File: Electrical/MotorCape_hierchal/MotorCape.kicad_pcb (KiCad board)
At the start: 2 copper layers, 24 parts, among them J1 Motor1, J10 DualMotorController_SIG, J11 flag_wheel servo, J12 Motor2, J13 Motor1, J14 DualMotorController_PWR, J16 DualMotorController_SIG, J17 Motor2, J2 DualMotorController_PWR, J4 DualMotorController_SIG, J5 Motor2, J6 Motor1, J7 i2c bus connector, J8 DualMotorController_PWR, P13 battery_connector, P14 Pi_Connector, U1 IMU

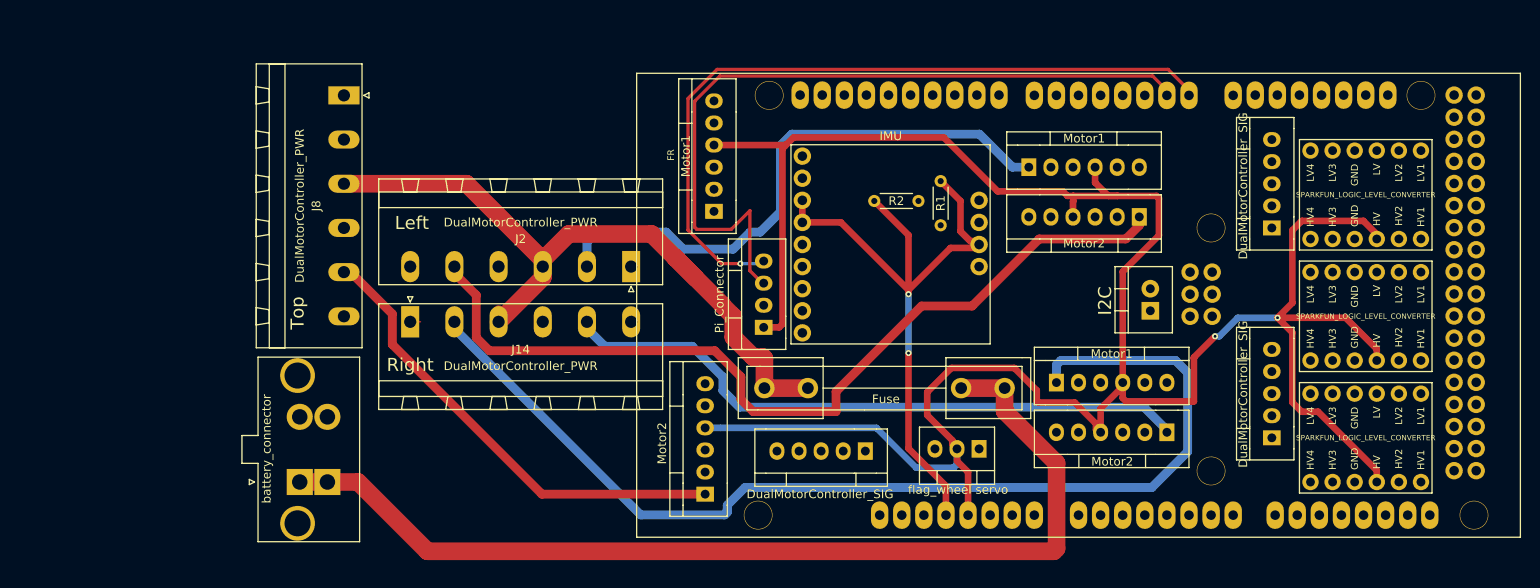
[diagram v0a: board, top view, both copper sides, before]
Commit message: pushing changes while routing. still not done yet
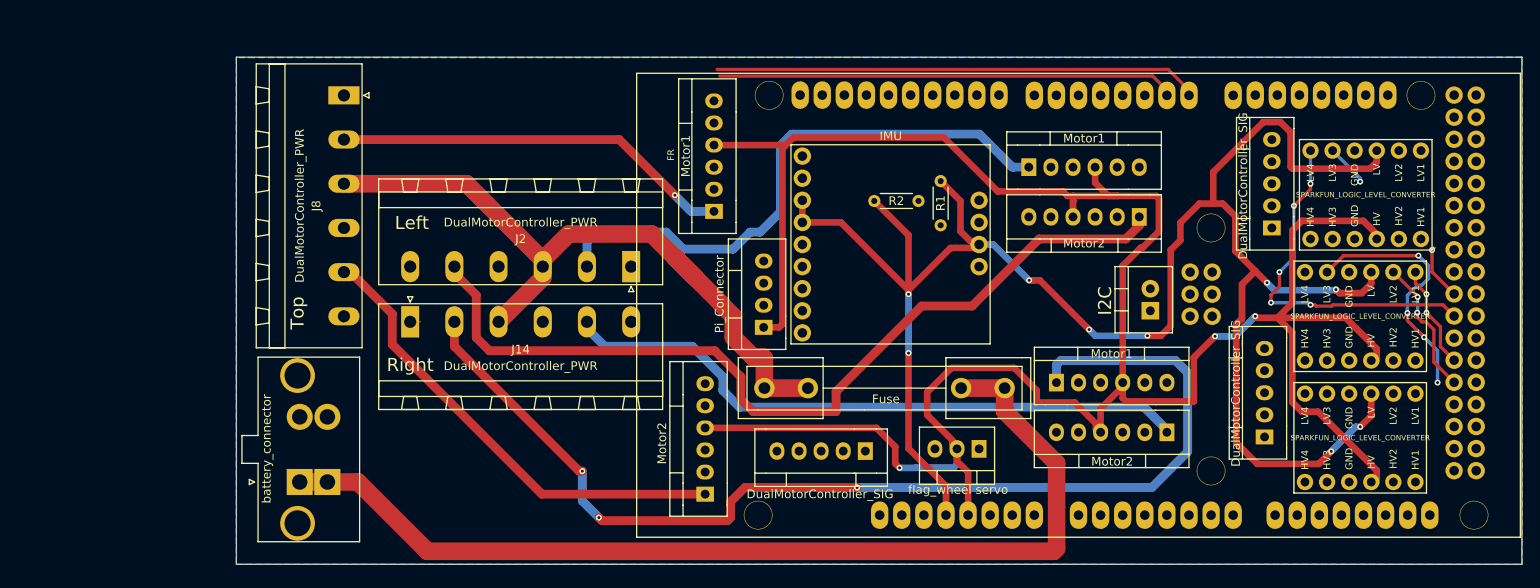
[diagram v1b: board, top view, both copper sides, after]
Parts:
- moved J16 0.84 mm to (183.9, 114.2)
- moved B1 0.63 mm to (192.4, 111.8)
- moved B2 0.63 mm to (192.4, 97.8)
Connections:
- ARD1 pad 54: FrontLeft_ENC_A -> Net-(ARD1-Pad54)
- ARD1 pad 55: FrontLeft_ENC_B -> FrontLeft_ENC_A
- ARD1 pad 56: BackLeft_DIR -> Net-(ARD1-Pad56)
- ARD1 pad 57: BackLeft_ENC_A -> FrontLeft_ENC_B
- ARD1 pad 58: BackLeft_ENC_B -> Net-(ARD1-Pad58)
- ARD1 pad 59: FrontRight_DIR -> BackLeft_DIR
- ARD1 pad 60: FrontRight_ENC_A -> Net-(ARD1-Pad60)
- ARD1 pad 61: FrontRight_ENC_B -> BackLeft_ENC_A
- ARD1 pad 62: BackRight_DIR -> Net-(ARD1-Pad62)
- ARD1 pad 63: BackRight_ENC_A -> BackLeft_ENC_B
- ARD1 pad 64: BackRight_ENC_B -> Net-(ARD1-Pad64)
- ARD1 pad 65: FlagWheel_DIR -> FrontRight_DIR
- ARD1 pad 66: FlagWheel_ENC_A -> Net-(ARD1-Pad66)
- ARD1 pad 67: FlagWheel_ENC_B -> FrontRight_ENC_A
- ARD1 pad 68: DrawBridge_DIR -> Net-(ARD1-Pad68)
- ARD1 pad 69: DrawBridge_ENC_A -> FrontRight_ENC_B
- ARD1 pad 70: DrawBridge_ENC_B -> Net-(ARD1-Pad70)
- ARD1 pad 71: Net-(ARD1-Pad71) -> BackRight_DIR
- ARD1 pad 73: Net-(ARD1-Pad73) -> BackRight_ENC_A
- ARD1 pad 75: Net-(ARD1-Pad75) -> BackRight_ENC_B
- ARD1 pad 77: Net-(ARD1-Pad77) -> FlagWheel_DIR
- ARD1 pad 79: Net-(ARD1-Pad79) -> FlagWheel_ENC_A
- ARD1 pad 81: Net-(ARD1-Pad81) -> FlagWheel_ENC_B
- ARD1 pad 82: Net-(ARD1-Pad82) -> DrawBridge_DIR
- ARD1 pad 83: Net-(ARD1-Pad83) -> DrawBridge_ENC_A
- ARD1 pad 84: Net-(ARD1-Pad84) -> DrawBridge_ENC_B
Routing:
- net +3V3: track 77.9 -> 221.4 mm, vias 2 -> 9
- net Net-(J6-Pad1): track 0.00 -> 47.6 mm, vias 0 -> 1
- net Tx_To_Pi: track 87.7 -> 52.8 mm
- net Rx_From_Pi: track 86.1 -> 56.2 mm, vias 1 -> 0
- net DrawBridge_ENC_A: track 0.00 -> 29.1 mm, vias 0 -> 4
- net BackRight_DIR: track 0.00 -> 28.1 mm, vias 0 -> 3
- net BackRight_ENC_B: track 0.00 -> 17.6 mm, vias 0 -> 2
- net FlagWheel_DIR: track 0.00 -> 9.54 mm
- net FlagWheel_ENC_A: track 0.00 -> 7.47 mm, vias 0 -> 2
- net FrontRight_ENC_B: track 0.00 -> 6.81 mm, vias 0 -> 1
- net FlagWheel_ENC_B: track 0.00 -> 6.33 mm, vias 0 -> 2
- net BackRight_ENC_A: track 0.00 -> 4.88 mm, vias 0 -> 1
- net Net-(J13-Pad1): track 125.7 -> 130.4 mm, vias 0 -> 3
- net +5V: track 277.0 -> 278.4 mm, vias 2 -> 3
- added copper zone on B.Cu, net MOTOR_GND
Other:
- board outline added: 147.8 x 58.3 mm

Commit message: pushing latest motor controller layout changes
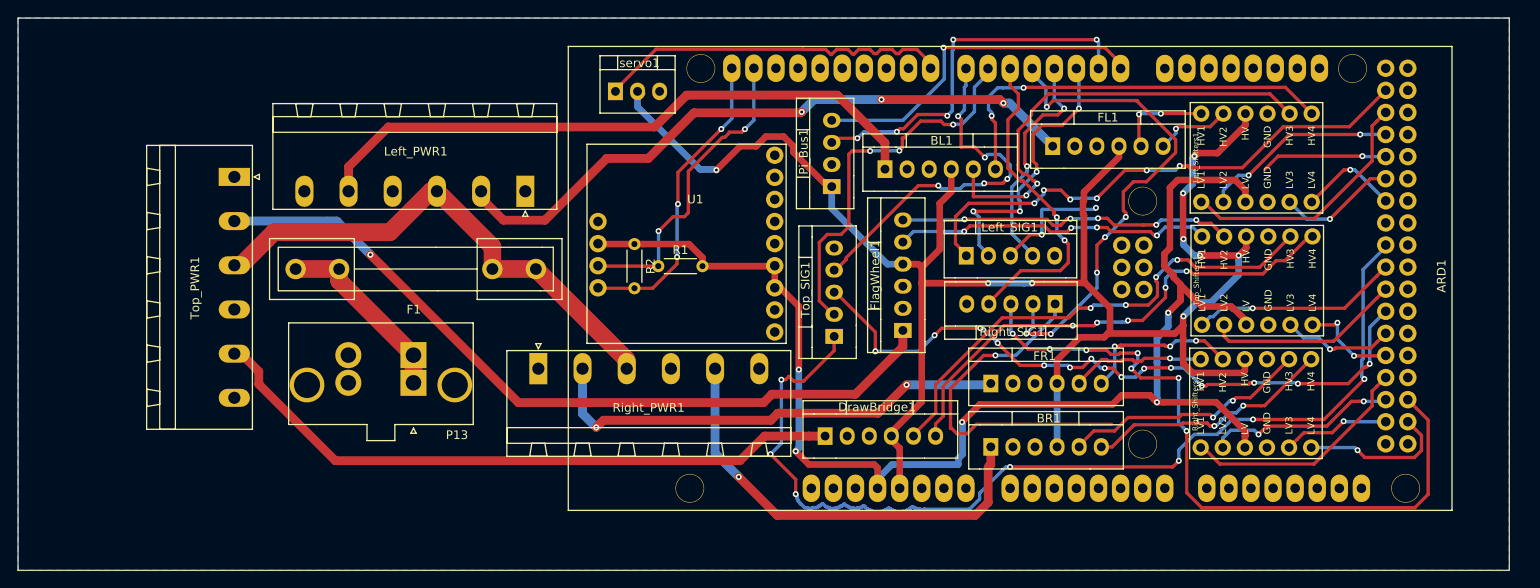
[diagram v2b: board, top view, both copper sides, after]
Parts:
- removed B1, B2, B3: SPARKFUN_LOGIC_LEVEL_CONVERTER, Sparkfun_Boards:SPARKFUN_LOGIC_LEVEL_CONVERTER
- removed J1, J13, J6: Motor1, MotorCapeComponents:Pin_Header_Latched_1x06
- removed J10, J16, J4: DualMotorController_SIG, MotorCapeComponents:Pin_Header_Latched_1x05
- removed J11: flag_wheel servo, MotorCapeComponents:Pin_Header_Latched_1x03
- removed J12, J17, J5: Motor2, MotorCapeComponents:Pin_Header_Latched_1x06
- removed J14, J2, J8: DualMotorController_PWR, Connectors_Phoenix:PhoenixContact_MSTBA-G_06x5.08mm_Angled
- removed J7: i2c bus connector, MotorCapeComponents:Pin_Header_Latched_1x02
- removed P14: Pi_Connector, MotorCapeComponents:Pin_Header_Latched_1x04
- added BL1: Motor2, MotorCapeComponents:Pin_Header_Latched_1x06, F.Cu at (135.2, 83.4)
- added BR1: Motor2, MotorCapeComponents:Pin_Header_Latched_1x06, F.Cu at (147.4, 115.3)
- added DrawBridge1: Motor2, MotorCapeComponents:Pin_Header_Latched_1x06, F.Cu at (128.3, 114.1)
- added FL1: Motor1, MotorCapeComponents:Pin_Header_Latched_1x06, F.Cu at (154.5, 80.8)
- added FR1: Motor1, MotorCapeComponents:Pin_Header_Latched_1x06, F.Cu at (147.4, 108.1)
- added FlagWheel1: Motor1, MotorCapeComponents:Pin_Header_Latched_1x06, F.Cu at (142.4, 102.0)
- added Left_PWR1: DualMotorController_PWR, Connectors_Phoenix:PhoenixContact_MSTBA-G_06x5.08mm_Angled, F.Cu at (96.4, 83.4)
- added Left_SIG1: DualMotorController_SIG, MotorCapeComponents:Pin_Header_Latched_1x05, F.Cu at (144.6, 93.4)
- added Left_Shifters1: SPARKFUN_LOGIC_LEVEL_CONVERTER, Sparkfun_Boards:SPARKFUN_LOGIC_LEVEL_CONVERTER, F.Cu at (180.5, 79.6)
- added Pi_Bus1: Pi_Connector, MotorCapeComponents:Pin_Header_Latched_1x04, F.Cu at (134.2, 85.4)
- added Right_PWR1: DualMotorController_PWR, Connectors_Phoenix:PhoenixContact_MSTBA-G_06x5.08mm_Angled, F.Cu at (97.9, 103.8)
- added Right_SIG1: DualMotorController_SIG, MotorCapeComponents:Pin_Header_Latched_1x05, F.Cu at (159.9, 93.8)
- added Right_Shifters1: SPARKFUN_LOGIC_LEVEL_CONVERTER, Sparkfun_Boards:SPARKFUN_LOGIC_LEVEL_CONVERTER, F.Cu at (180.4, 107.8)
- added Top_PWR1: DualMotorController_PWR, Connectors_Phoenix:PhoenixContact_MSTBA-G_06x5.08mm_Angled, F.Cu at (63.0, 81.8)
- added Top_SIG1: DualMotorController_SIG, MotorCapeComponents:Pin_Header_Latched_1x05, F.Cu at (134.5, 102.6)
- added Top_Shifters1: SPARKFUN_LOGIC_LEVEL_CONVERTER, Sparkfun_Boards:SPARKFUN_LOGIC_LEVEL_CONVERTER, F.Cu at (180.6, 93.7)
- added servo1: flag_wheel servo, MotorCapeComponents:Pin_Header_Latched_1x03, F.Cu at (105.0, 74.4)
- moved U1 51.7 mm to (103.5, 78.0), turned to 0 degrees
- moved R1 32.8 mm to (111.7, 92.0), turned to 0 degrees
- moved F1 29.6 mm to (97.6, 92.4), turned to 180 degrees
- moved R2 28.0 mm to (109.0, 89.5), turned to 270 degrees
- moved P13 17.4 mm to (83.6, 105.4), turned to 180 degrees
- moved ARD1 8.45 mm to (101.4, 66.8)
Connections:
- ARD1 pad 67: FrontRight_ENC_A -> FlagWheel_DIR
- ARD1 pad 69: FrontRight_ENC_B -> FlagWheel_ENC_A
- ARD1 pad 71: BackRight_DIR -> FlagWheel_ENC_B
- ARD1 pad 73: BackRight_ENC_A -> DrawBridge_DIR
- ARD1 pad 75: BackRight_ENC_B -> DrawBridge_ENC_A
- ARD1 pad 77: FlagWheel_DIR -> DrawBridge_ENC_B
- ARD1 pad 79: FlagWheel_ENC_A -> FrontRight_ENC_A
- ARD1 pad 81: FlagWheel_ENC_B -> FrontRight_ENC_B
- ARD1 pad 82: DrawBridge_DIR -> BackRight_DIR
- ARD1 pad 83: DrawBridge_ENC_A -> BackRight_ENC_A
- ARD1 pad 84: DrawBridge_ENC_B -> BackRight_ENC_B
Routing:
- net Net-(J13-Pad1): track 130.4 -> 0.00 mm, vias 3 -> 0
- net FlagWheel_DIR: track 9.54 -> 116.8 mm, vias 0 -> 7
- net Net-(J2-Pad5): track 103.2 -> 0.00 mm
- net +12V: track 116.4 -> 21.6 mm
- net Net-(FlagWheel1-Pad1): track 0.00 -> 90.0 mm, vias 0 -> 1
- net DrawBridge_DIR: track 0.00 -> 79.2 mm, vias 0 -> 15
- net Net-(FL1-Pad1): track 0.00 -> 75.5 mm, vias 0 -> 3
- net Net-(DrawBridge1-Pad1): track 0.00 -> 75.0 mm
- net Net-(J14-Pad5): track 74.4 -> 0.00 mm
- net Net-(BL1-Pad1): track 0.00 -> 73.3 mm
- net Net-(J1-Pad1): track 67.9 -> 0.00 mm
- net +5V: track 278.4 -> 212.7 mm, vias 3 -> 10
- net FrontLeft_DIR: track 0.00 -> 61.8 mm, vias 0 -> 6
- net +3V3: track 221.4 -> 159.8 mm, vias 9 -> 5
- net FrontRight_SPD: track 0.00 -> 58.3 mm, vias 0 -> 6
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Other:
- board size 147.8 x 58.3 mm -> 171.5 x 63.5 mm
- board text removed: "FR"
- board text removed: "I2C"
- board text removed: "Left"
- board text removed: "Right"
- board text removed: "Top"
